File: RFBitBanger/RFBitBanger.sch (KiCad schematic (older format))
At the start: 86 parts, among them J1 POWER, J11 SPEAKER, J13 Conn_01x01, J14 Conn_01x01, J15 Conn_01x01, J16 Conn_01x01, J2 Barrel_Jack, J20 Conn_01x01, J21 Conn_01x01, J3 Conn_01x01, J4 Conn_01x01, J5 Conn_01x04, J6 Conn_01x01, J7 Conn_01x01, J8 Conn_01x01, J9 ICSP, P1 Mini-DIN_6pins_ver4, Q14 2N3904, Q4 2N3904, SW1 SW_Push, SW2 SW_Push, SW3 SW_Push, SW4 SW_Push, SW5 SW_Push, T4 Common-Mode Choke, U1 ATMEGA328-PU, U2 LM7805_TO220, U3 LM386, U5 LCD1602ExtraPins, Y1 16 MHz

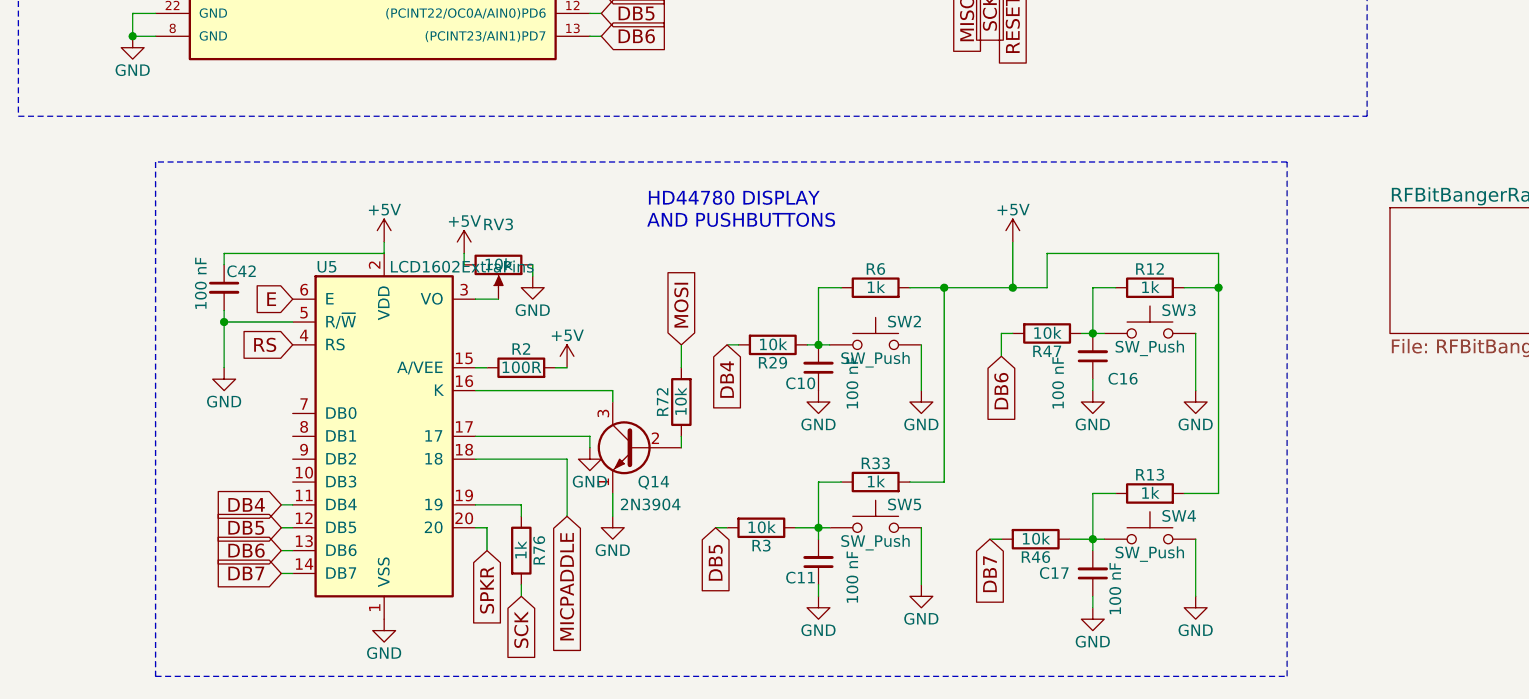
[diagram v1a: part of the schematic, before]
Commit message: Added fifth button
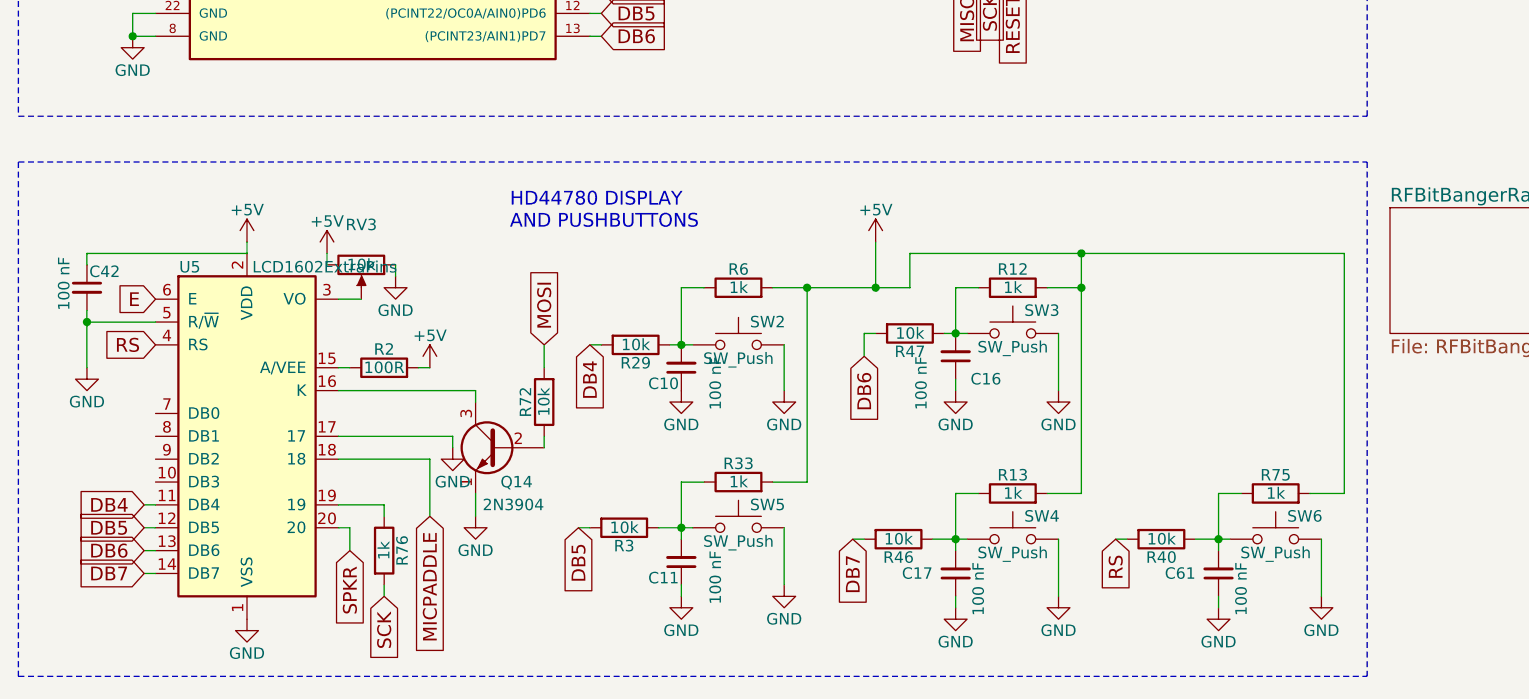
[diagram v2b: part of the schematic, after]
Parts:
- added C61: 100 nF, Capacitors_THT:C_Disc_D5.0mm_W2.5mm_P2.50mm, symbol C_Small
- added R40: 10k, Resistors_THT:R_Axial_DIN0207_L6.3mm_D2.5mm_P7.62mm_Horizontal, symbol R
- added R75: 1k, Resistors_THT:R_Axial_DIN0207_L6.3mm_D2.5mm_P7.62mm_Horizontal, symbol R
- added SW6: SW_Push, Buttons_Switches_THT:SW_PUSH_6mm, symbol SW_Push
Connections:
- net +5V: now also R75.2
- net GND: now also C61.1, SW6.2
- net RS: now also R40.2
- new net: C61.2, R40.1, R75.1, SW6.1
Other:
- moved on the sheet: C10, C11, C16, C17, C42, Q14, R12, R13, R2, R29, R3, R33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
